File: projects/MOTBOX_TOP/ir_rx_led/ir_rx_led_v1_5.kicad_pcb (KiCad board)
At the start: 2 copper layers, 11.9 x 32 mm, 5 parts, among them J1 Conn_01x03

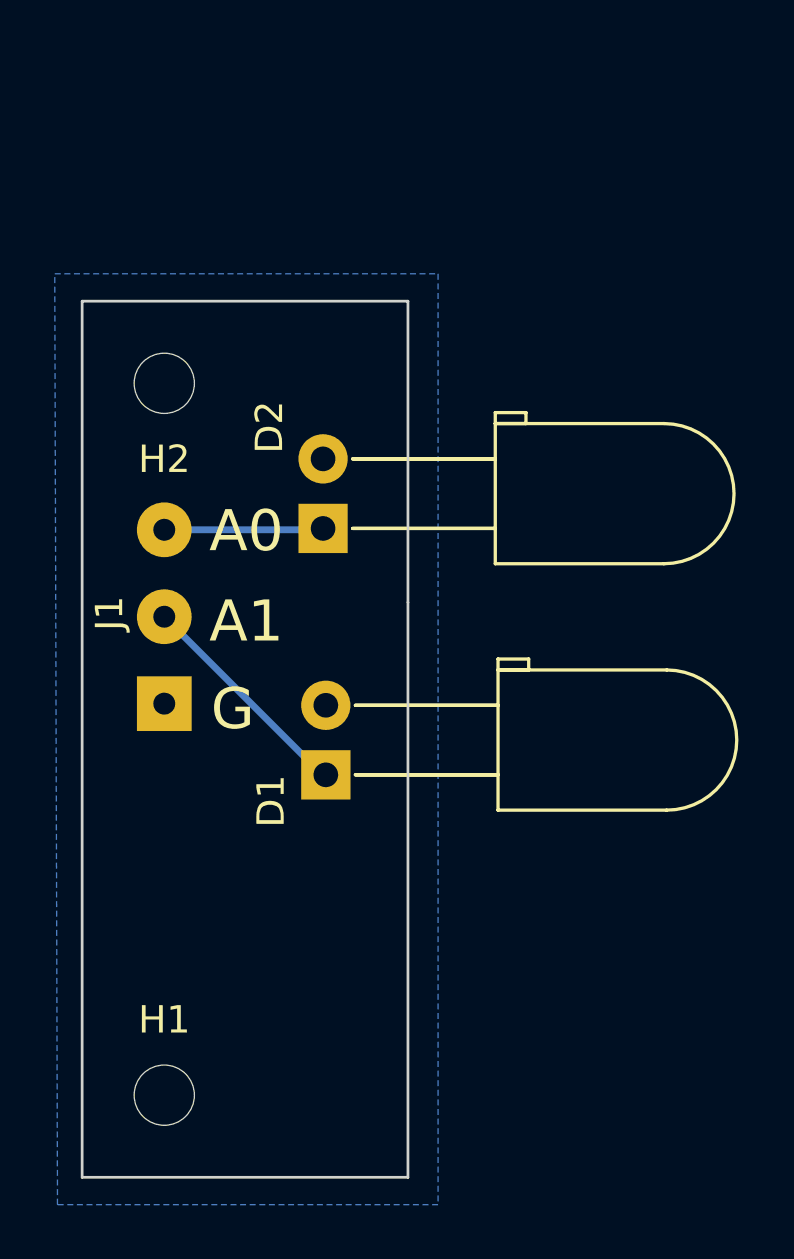
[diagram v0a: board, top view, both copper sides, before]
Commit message: Modified v1_5
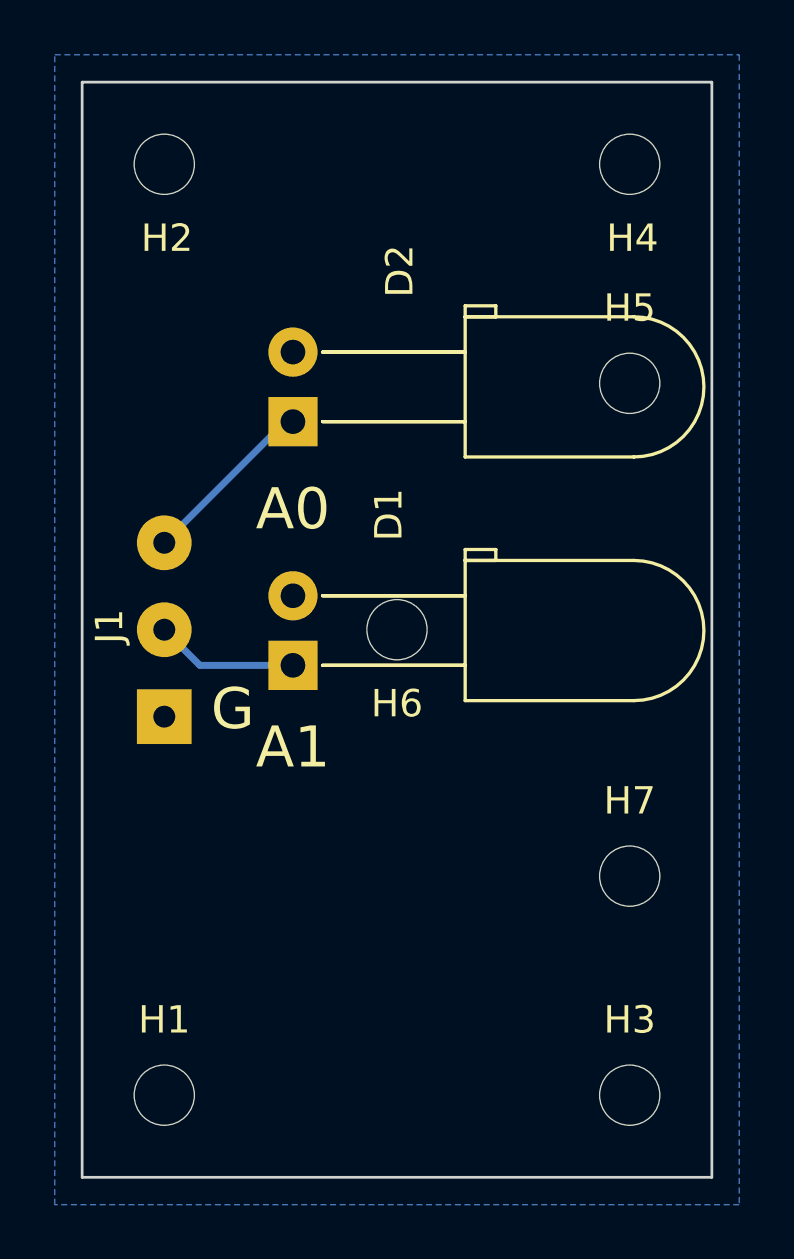
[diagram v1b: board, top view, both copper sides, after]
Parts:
- added H3: MountingHole, MountingHole:MountingHole_2.2mm_M2_ISO7380, F.Cu at (150.0, 68.0)
- added H4: MountingHole, MountingHole:MountingHole_2.2mm_M2_ISO7380, F.Cu at (150.0, 34.0)
- added H5: MountingHole, MountingHole:MountingHole_2.2mm_M2_ISO7380, F.Cu at (150.0, 42.0)
- added H6: MountingHole, MountingHole:MountingHole_2.2mm_M2_ISO7380, F.Cu at (141.5, 51.0)
- added H7: MountingHole, MountingHole:MountingHole_2.2mm_M2_ISO7380, F.Cu at (150.0, 60.0)
- H1: value MountingHole -> MountingHole
- moved H2 8.00 mm to (133.0, 34.0)
- moved D1 4.18 mm to (137.7, 52.3)
- moved D2 4.05 mm to (137.7, 43.4)
- moved J1 0.47 mm to (133.0, 54.2)
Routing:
- net Net-(D1-Pad1): track 8.29 -> 5.24 mm
- net Net-(D2-Pad1): track 5.82 -> 6.53 mm
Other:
- board size 11.9 x 32 mm -> 23 x 40 mm
